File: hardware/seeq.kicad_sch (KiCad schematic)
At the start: 87 parts, among them J1 MIDI IN, J2 AudioJack2_SwitchT, J3 Conn_01x06, J4 Conn_01x04, J5 AudioJack2_SwitchT, J6 MIDI OUT, SW1 SW_DIP_x01, SW10 SW_DIP_x01, SW11 SW_DIP_x01, SW12 SW_DIP_x01, SW13 SW_DIP_x01, SW14 SW_DIP_x01, SW15 SW_DIP_x01, SW16 SW_DIP_x01, SW17 RotaryEncoder_Switch, SW2 SW_DIP_x01, SW3 SW_DIP_x01, SW4 SW_DIP_x01, SW5 SW_DIP_x01, SW6 SW_DIP_x01, SW7 SW_DIP_x01, SW8 SW_DIP_x01, SW9 SW_DIP_x01, U1 6N138, U2 Pico

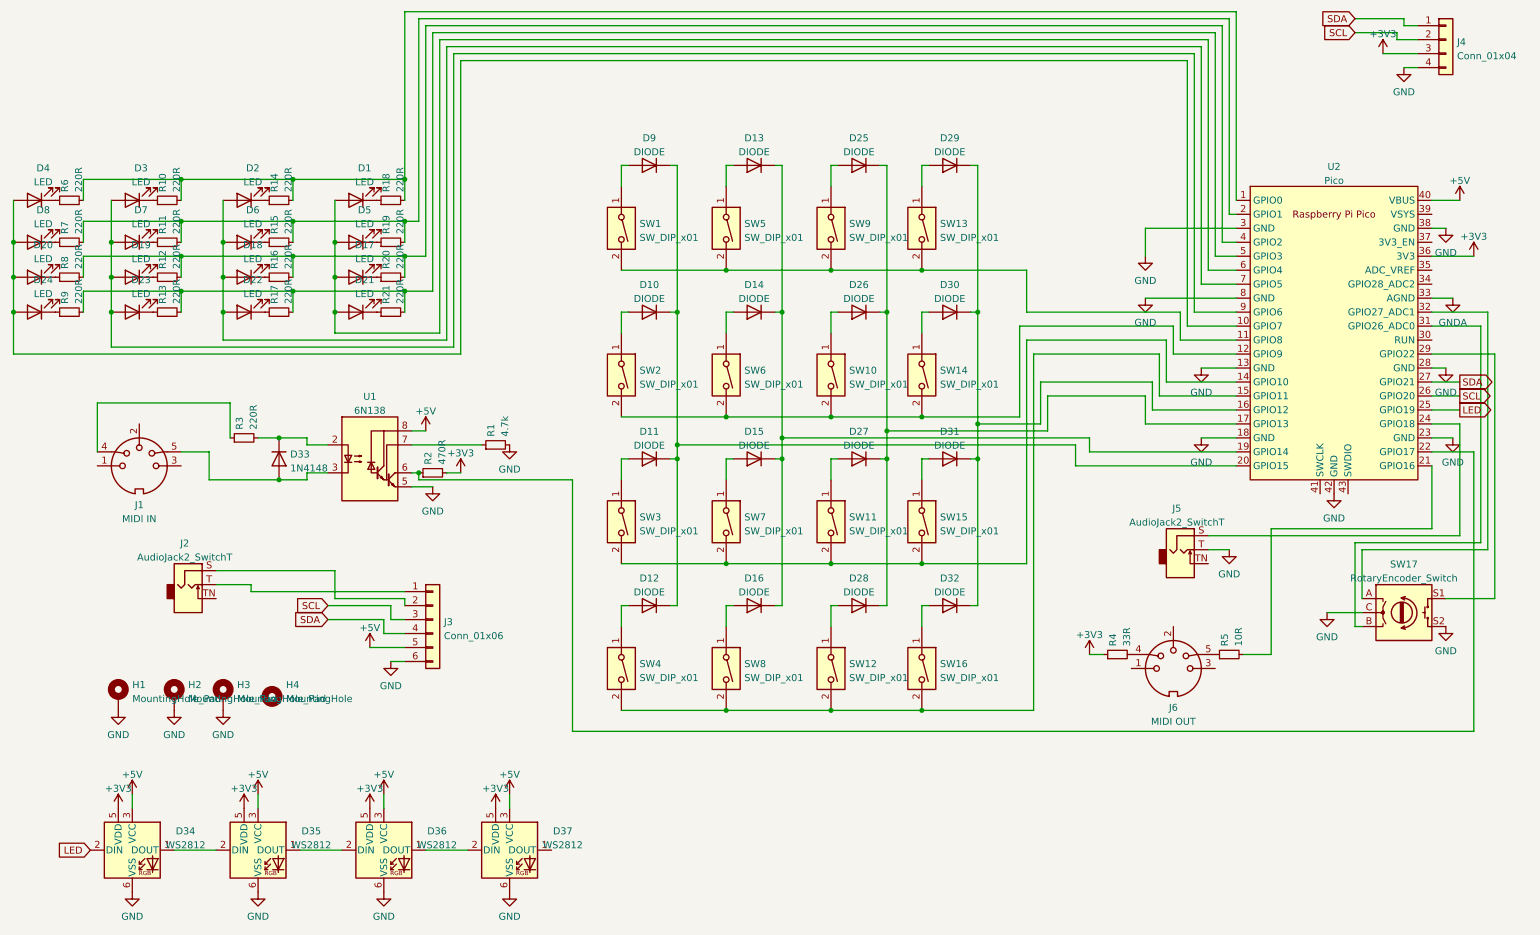
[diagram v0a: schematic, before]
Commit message: Update software for PCB + PCB fixes
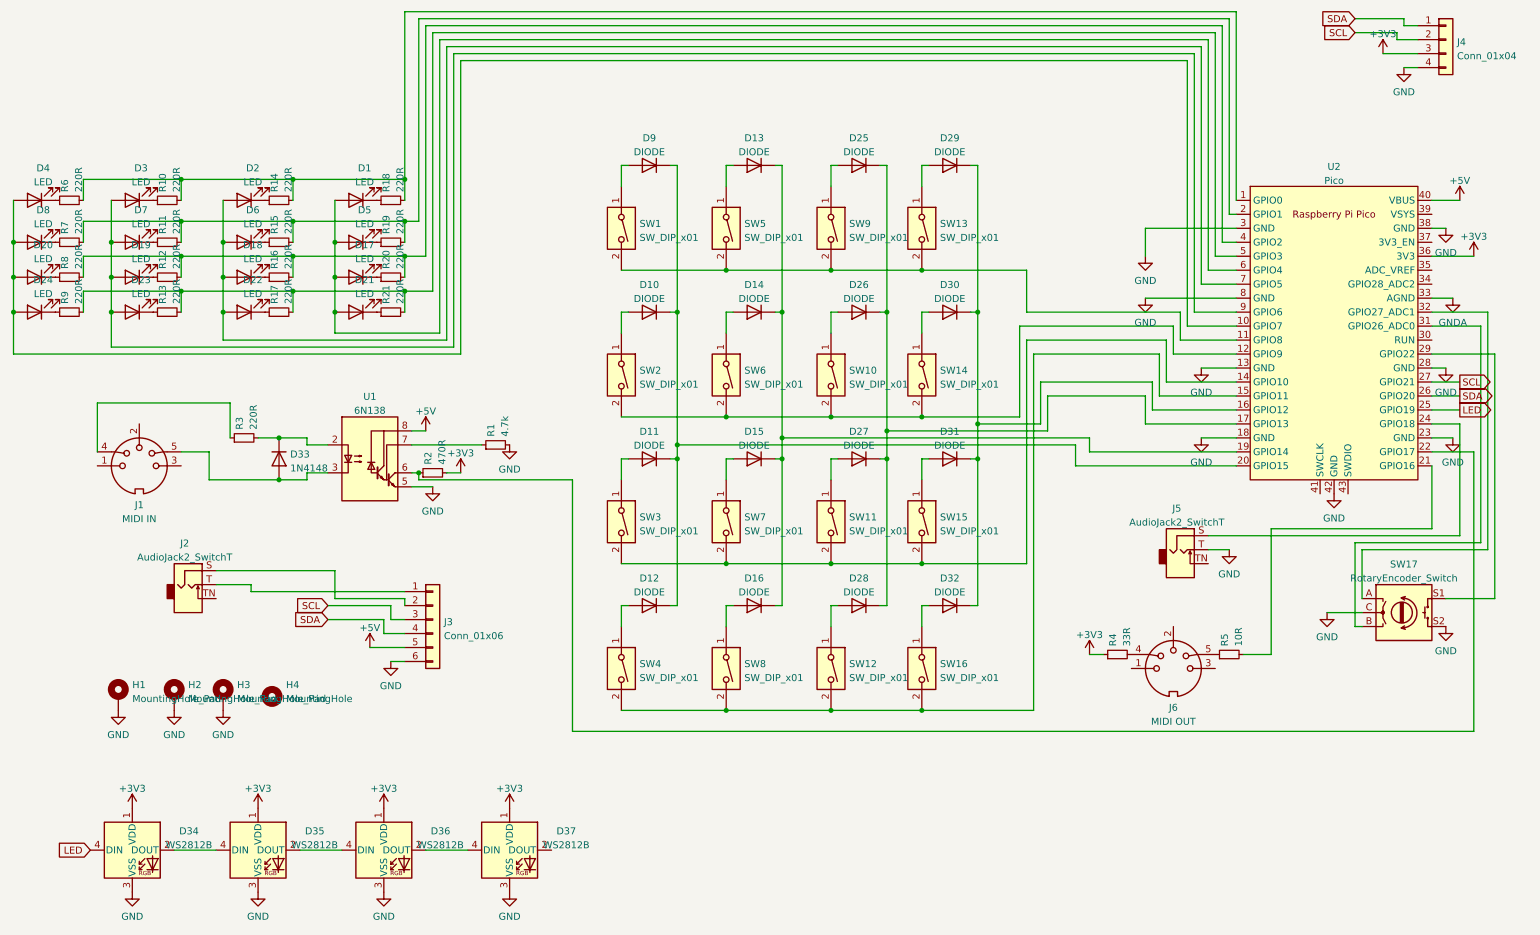
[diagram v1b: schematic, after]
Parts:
- removed D34, D35, D36, D37: WS2812, LED_SMD:LED_WS2812_PLCC6_5.0x5.0mm_P1.6mm, symbol LED:WS2812
- added D34, D35, D36, D37: WS2812B, LED_SMD:LED_WS2812B_PLCC4_5.0x5.0mm_P3.2mm, symbol LED:WS2812B
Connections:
- net +3V3: now also D34.1 (VDD), D35.1 (VDD), D36.1 (VDD), D37.1 (VDD)
- net GND: now also D34.3 (VSS), D35.3 (VSS), D36.3 (VSS), D37.3 (VSS)
- net LED: now also D34.4 (DIN)
- net SCL: now also U2.27 (GPIO21); no longer U2.26 (GPIO20)
- net SDA: now also U2.26 (GPIO20); no longer U2.27 (GPIO21)
- new net: D36.2 (DOUT), D37.4 (DIN)
- new net: D35.2 (DOUT), D36.4 (DIN)
- new net: D34.2 (DOUT), D35.4 (DIN)
